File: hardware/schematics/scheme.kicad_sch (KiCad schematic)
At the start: 10 parts

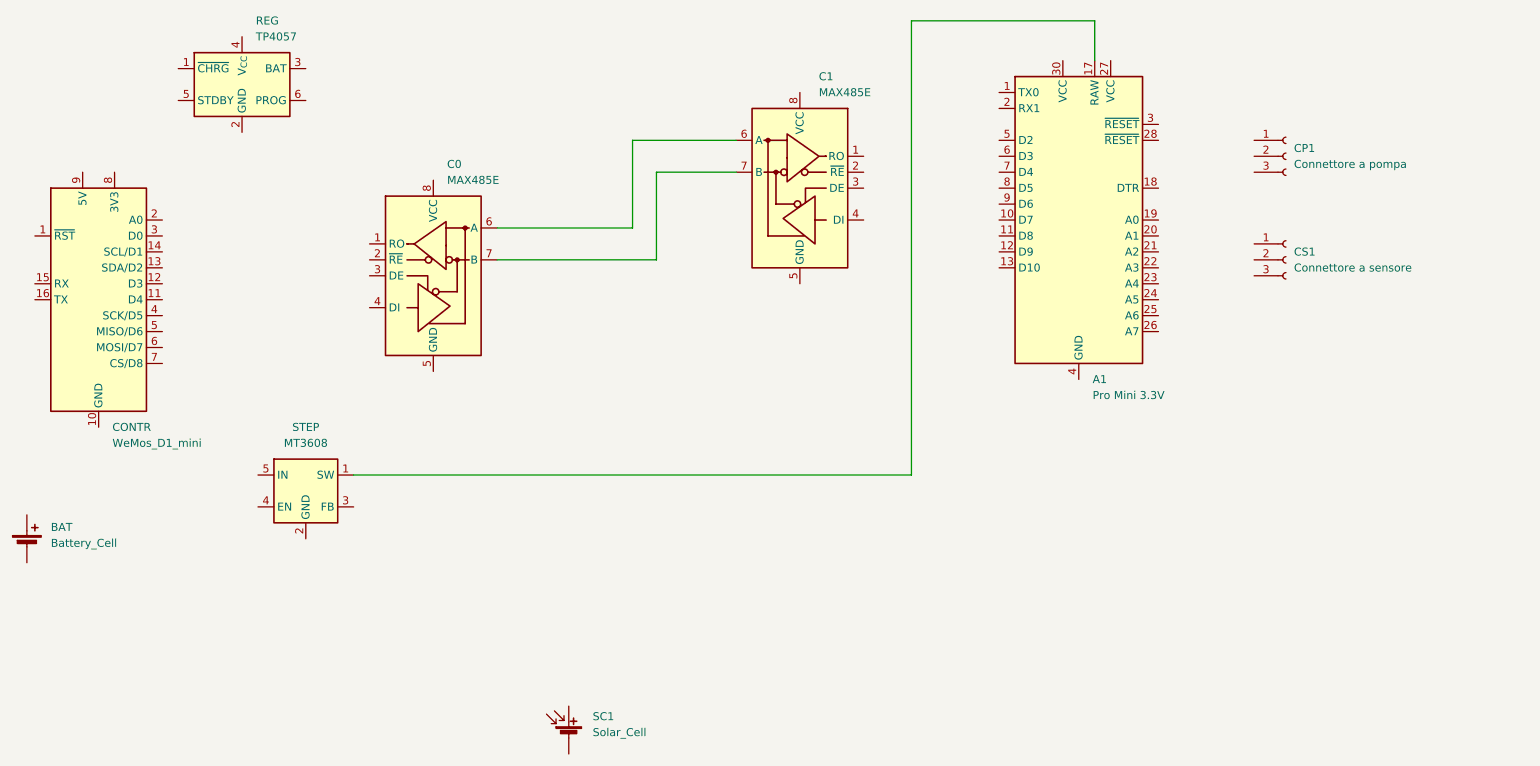
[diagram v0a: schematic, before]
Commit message: changed schema
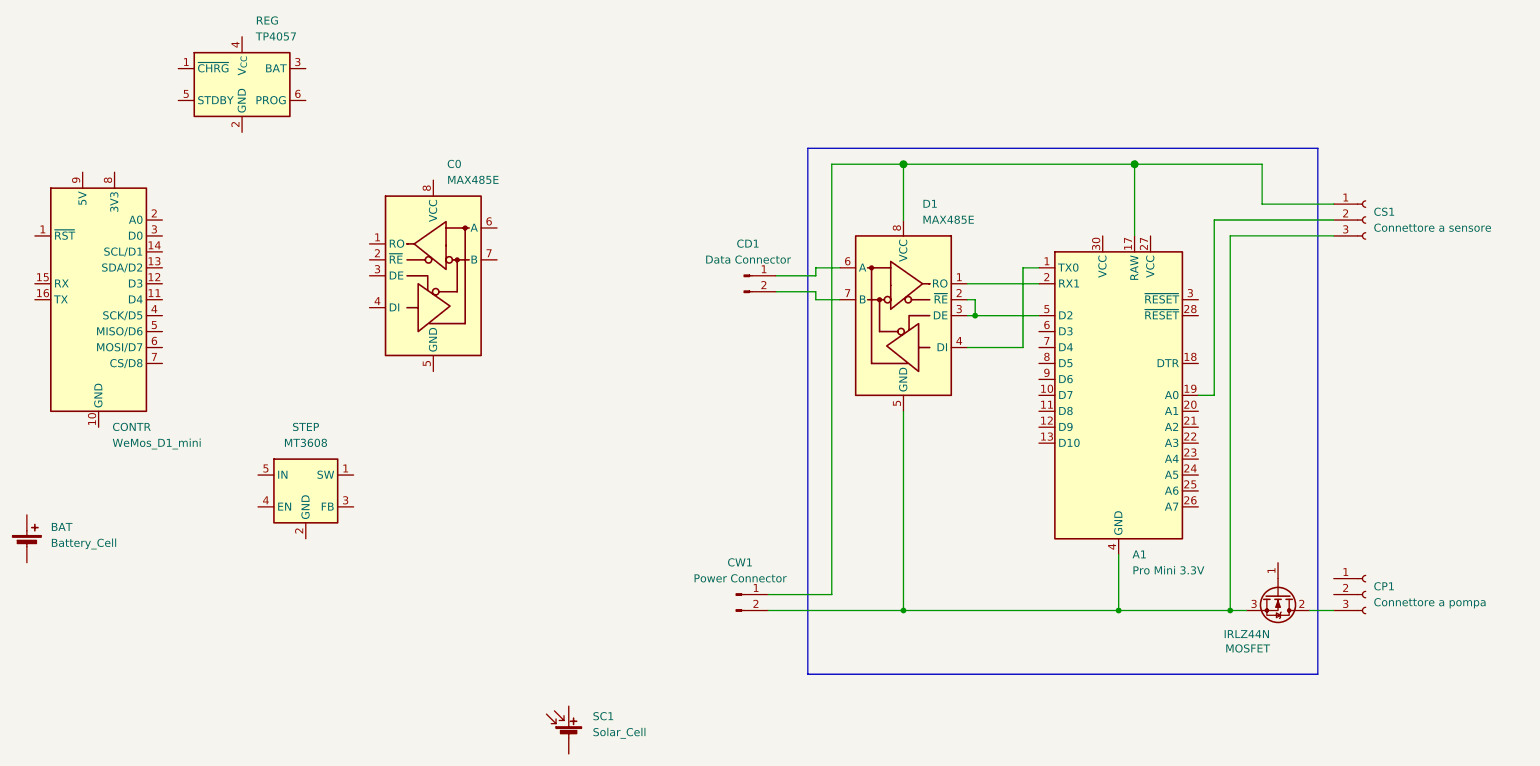
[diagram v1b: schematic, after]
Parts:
- added CD1: Data Connector, symbol Connector:Conn_01x02_Pin
- added CW1: Power Connector, symbol Connector:Conn_01x02_Pin
- added MOSFET: IRLZ44N, Package_TO_SOT_THT:TO-220-3_Vertical, symbol Transistor_FET:IRLZ44N
- renumbered C1 to D1
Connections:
- net at CP1.3 (Pin_3): now also MOSFET.2 (D)
- net at STEP.1 (SW): no longer A1.17 (RAW)
- net at D1.1 (RO): now also A1.2 (RX1)
- net at D1.2 (~{RE}): now also A1.5 (D2), D1.3 (DE)
- net at D1.4 (DI): now also A1.1 (TX0)
- net at D1.5 (GND): now also A1.29 (GND), A1.4 (GND), CS1.3 (Pin_3), CW1.2 (Pin_2), MOSFET.3 (S)
- net at D1.6 (A): now also CD1.1 (Pin_1); no longer C0.6 (A)
- net at D1.7 (B): now also CD1.2 (Pin_2); no longer C0.7 (B)
- net at D1.8 (VCC): now also A1.17 (RAW), CS1.1 (Pin_1), CW1.1 (Pin_1)
- net at CS1.2 (Pin_2): now also A1.19 (A0)
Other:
- moved on the sheet: A1, CP1, CS1, D1
